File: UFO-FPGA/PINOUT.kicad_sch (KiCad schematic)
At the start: 4 parts, among them J1 Power, J2 Digital, J3 Digital/PWM, J4 Digital

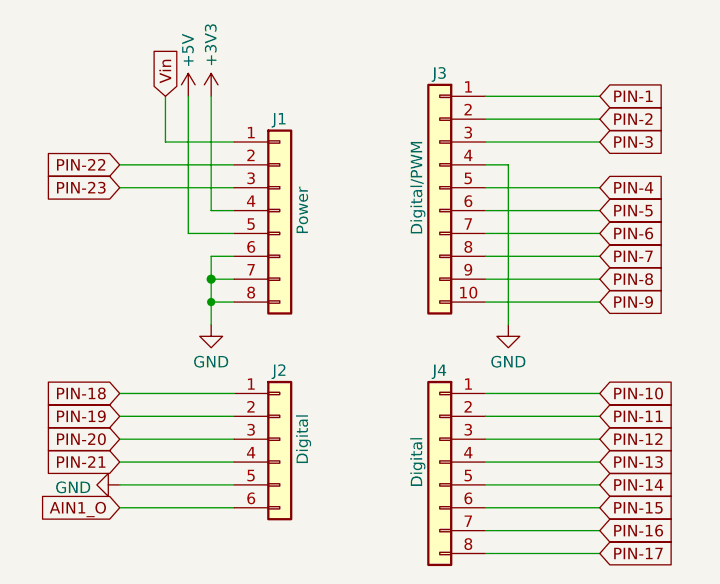
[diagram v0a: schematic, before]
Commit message: pcb prog redesign
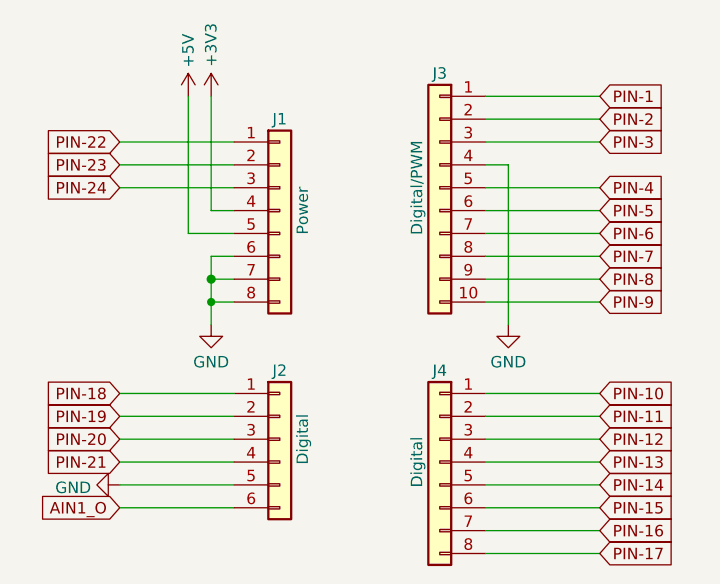
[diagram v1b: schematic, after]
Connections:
- net Vin is gone; now on net PIN-22: J1.1 (Pin_1)
- net PIN-22: no longer J1.2 (Pin_2)
- net PIN-23: now also J1.2 (Pin_2); no longer J1.3 (Pin_3)
- new net PIN-24: J1.3 (Pin_3)
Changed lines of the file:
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@@
     (stroke (width 0) (type solid))
-  )
-  (wire (pts (xy 116.84 64.77) (xy 124.46 64.77))
-    (stroke (width 0) (type default))
   )
   (wire (pts (xy 152.4 105.41) (xy 165.1 105.41))
@@
     (stroke (width 0) (type solid))
   )
-  (wire (pts (xy 116.84 64.77) (xy 116.84 59.69))
-    (stroke (width 0) (type solid))
-  )
   (wire (pts (xy 111.76 67.31) (xy 124.46 67.31))
     (stroke (width 0) (type default))
@@
     (stroke (width 0) (type solid))
   )
+  (wire (pts (xy 111.76 64.77) (xy 124.46 64.77))
+    (stroke (width 0) (type default))
+  )
   (wire (pts (xy 152.4 80.01) (xy 165.1 80.01))
     (stroke (width 0) (type solid))
@@
     )
   )
-  (global_label "PIN-23" (shape input) (at 111.76 69.85 180) (fields_autoplaced)
+  (global_label "PIN-23" (shape input) (at 111.76 67.31 180) (fields_autoplaced)
+    (effects (font (size 1.27 1.27)) (justify right))
+    (property "Intersheetrefs" "${INTERSHEET_REFS}" (at 101.6575 67.31 0)
+      (effects (font (size 1.27 1.27)) (justify right) hide)
+    )
+  )
+  (global_label "PIN-3" (shape input) (at 165.1 64.77 0) (fields_autoplaced)
+    (effects (font (size 1.27 1.27)) (justify left))
+    (property "Intersheetrefs" "${INTERSHEET_REFS}" (at 173.993 64.77 0)
+      (effects (font (size 1.27 1.27)) (justify left) hide)
+    )
+  )
+  (global_label "PIN-17" (shape input) (at 165.1 110.49 0) (fields_autoplaced)
+    (effects (font (size 1.27 1.27)) (justify left))
+    (property "Intersheetrefs" "${INTERSHEET_REFS}" (at 175.2025 110.49 0)
+      (effects (font (size 1.27 1.27)) (justify left) hide)
+    )
+  )
+  (global_label "PIN-4" (shape input) (at 165.1 69.85 0) (fields_autoplaced)
+    (effects (font (size 1.27 1.27)) (justify left))
+    (property "Intersheetrefs" "${INTERSHEET_REFS}" (at 173.993 69.85 0)
+      (effects (font (size 1.27 1.27)) (justify left) hide)
+    )
+  )
+  (global_label "PIN-1" (shape input) (at 165.1 59.69 0) (fields_autoplaced)
+    (effects (font (size 1.27 1.27)) (justify left))
+    (property "Intersheetrefs" "${INTERSHEET_REFS}" (at 173.993 59.69 0)
+      (effects (font (size 1.27 1.27)) (justify left) hide)
+    )
+  )
+  (global_label "PIN-20" (shape input) (at 111.76 97.79 180) (fields_autoplaced)
+    (effects (font (size 1.27 1.27)) (justify right))
+    (property "Intersheetrefs" "${INTERSHEET_REFS}" (at 101.6575 97.79 0)
+      (effects (font (size 1.27 1.27)) (justify right) hide)
+    )
+  )
+  (global_label "PIN-10" (shape input) (at 165.1 92.71 0) (fields_autoplaced)
+    (effects (font (size 1.27 1.27)) (justify left))
+    (property "Intersheetrefs" "${INTERSHEET_REFS}" (at 175.2025 92.71 0)
+      (effects (font (size 1.27 1.27)) (justify left) hide)
+    )
+  )
+  (global_label "PIN-11" (shape input) (at 165.1 95.25 0) (fields_autoplaced)
+    (effects (font (size 1.27 1.27)) (justify left))
+    (property "Intersheetrefs" "${INTERSHEET_REFS}" (at 175.2025 95.25 0)
+      (effects (font (size 1.27 1.27)) (justify left) hide)
+    )
+  )
+  (global_label "PIN-13" (shape input) (at 165.1 100.33 0) (fields_autoplaced)
+    (effects (font (size 1.27 1.27)) (justify left))
+    (property "Intersheetrefs" "${INTERSHEET_REFS}" (at 175.2025 100.33 0)
+      (effects (font (size 1.27 1.27)) (justify left) hide)
+    )
+  )
+  (global_label "PIN-24" (shape input) (at 111.76 69.85 180) (fields_autoplaced)
     (effects (font (size 1.27 1.27)) (justify right))
     (property "Intersheetrefs" "${INTERSHEET_REFS}" (at 101.6575 69.85 0)
@@
     )
   )
-  (global_label "PIN-3" (shape input) (at 165.1 64.77 0) (fields_autoplaced)
-    (effects (font (size 1.27 1.27)) (justify left))
-    (property "Intersheetrefs" "${INTERSHEET_REFS}" (at 173.993 64.77 0)
-      (effects (font (size 1.27 1.27)) (justify left) hide)
-    )
-  )
-  (global_label "PIN-17" (shape input) (at 165.1 110.49 0) (fields_autoplaced)
-    (effects (font (size 1.27 1.27)) (justify left))
-    (property "Intersheetrefs" "${INTERSHEET_REFS}" (at 175.2025 110.49 0)
-      (effects (font (size 1.27 1.27)) (justify left) hide)
-    )
-  )
-  (global_label "PIN-4" (shape input) (at 165.1 69.85 0) (fields_autoplaced)
-    (effects (font (size 1.27 1.27)) (justify left))
-    (property "Intersheetrefs" "${INTERSHEET_REFS}" (at 173.993 69.85 0)
-      (effects (font (size 1.27 1.27)) (justify left) hide)
-    )
-  )
-  (global_label "PIN-1" (shape input) (at 165.1 59.69 0) (fields_autoplaced)
-    (effects (font (size 1.27 1.27)) (justify left))
-    (property "Intersheetrefs" "${INTERSHEET_REFS}" (at 173.993 59.69 0)
-      (effects (font (size 1.27 1.27)) (justify left) hide)
-    )
-  )
-  (global_label "PIN-20" (shape input) (at 111.76 97.79 180) (fields_autoplaced)
-    (effects (font (size 1.27 1.27)) (justify right))
-    (property "Intersheetrefs" "${INTERSHEET_REFS}" (at 101.6575 97.79 0)
-      (effects (font (size 1.27 1.27)) (justify right) hide)
-    )
-  )
-  (global_label "PIN-10" (shape input) (at 165.1 92.71 0) (fields_autoplaced)
-    (effects (font (size 1.27 1.27)) (justify left))
-    (property "Intersheetrefs" "${INTERSHEET_REFS}" (at 175.2025 92.71 0)
-      (effects (font (size 1.27 1.27)) (justify left) hide)
-    )
-  )
-  (global_label "PIN-11" (shape input) (at 165.1 95.25 0) (fields_autoplaced)
-    (effects (font (size 1.27 1.27)) (justify left))
-    (property "Intersheetrefs" "${INTERSHEET_REFS}" (at 175.2025 95.25 0)
-      (effects (font (size 1.27 1.27)) (justify left) hide)
-    )
-  )
-  (global_label "PIN-13" (shape input) (at 165.1 100.33 0) (fields_autoplaced)
-    (effects (font (size 1.27 1.27)) (justify left))
-    (property "Intersheetrefs" "${INTERSHEET_REFS}" (at 175.2025 100.33 0)
-      (effects (font (size 1.27 1.27)) (justify left) hide)
-    )
-  )
   (global_label "PIN-15" (shape input) (at 165.1 105.41 0) (fields_autoplaced)
     (effects (font (size 1.27 1.27)) (justify left))
@@
     )
   )
-  (global_label "Vin" (shape input) (at 116.84 59.69 90) (fields_autoplaced)
-    (effects (font (size 1.27 1.27)) (justify left))
-    (property "Intersheetrefs" "${INTERSHEET_REFS}" (at 116.84 53.9418 90)
-      (effects (font (size 1.27 1.27)) (justify left) hide)
-    )
-  )
   (global_label "PIN-7" (shape input) (at 165.1 77.47 0) (fields_autoplaced)
     (effects (font (size 1.27 1.27)) (justify left))
@@
     )
   )
-  (global_label "PIN-22" (shape input) (at 111.76 67.31 180) (fields_autoplaced)
-    (effects (font (size 1.27 1.27)) (justify right))
-    (property "Intersheetrefs" "${INTERSHEET_REFS}" (at 101.6575 67.31 0)
-      (effects (font (size 1.27 1.27)) (justify right) hide)
-    )
+  (global_label "PIN-22" (shape input) (at 111.76 64.77 180) (fields_autoplaced)
+    (effects (font (size 1.27 1.27)) (justify right))
+    (property "Intersheetrefs" "${INTERSHEET_REFS}" (at 101.6575 64.77 0)
+      (effects (font (size 1.27 1.27)) (justify right) hide)
+    )
